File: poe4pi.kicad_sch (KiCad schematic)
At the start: 30 parts, among them J1 Conn_02x02_Odd_Even, J2 Conn_02x02_Odd_Even, J3 Conn_02x20_Odd_Even, U1 LTC4413EDD-2-PBF, U3 TPS2375-1

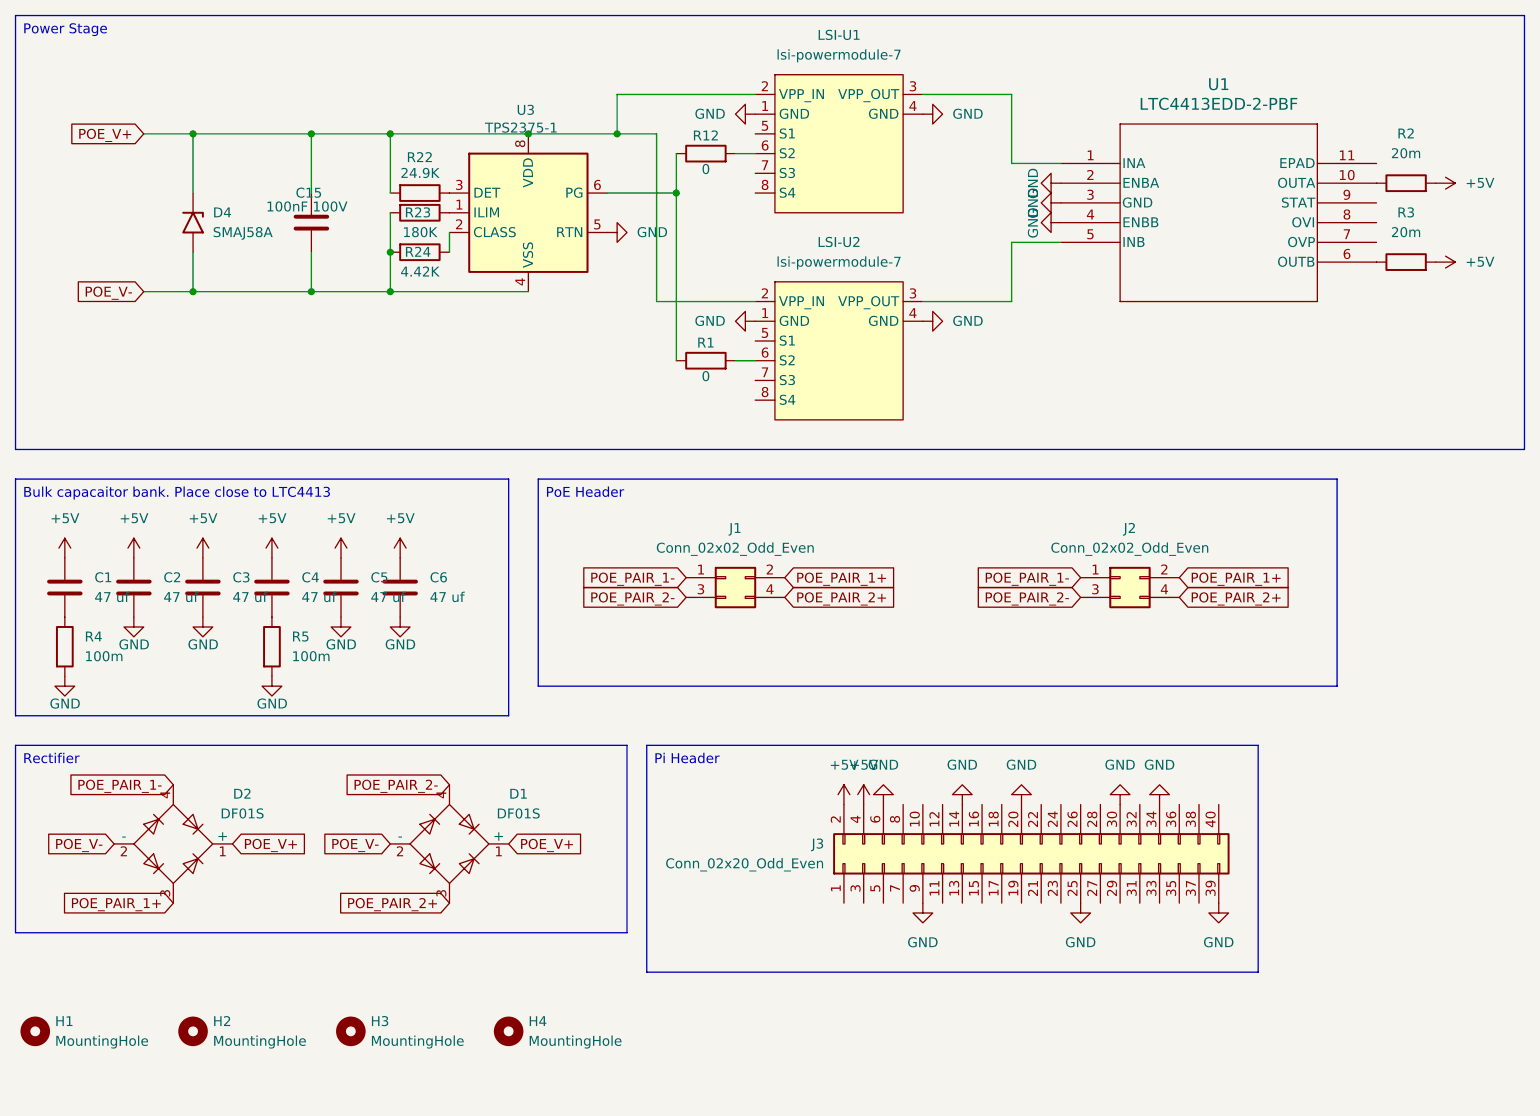
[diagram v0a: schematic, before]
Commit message: feat: v0.1
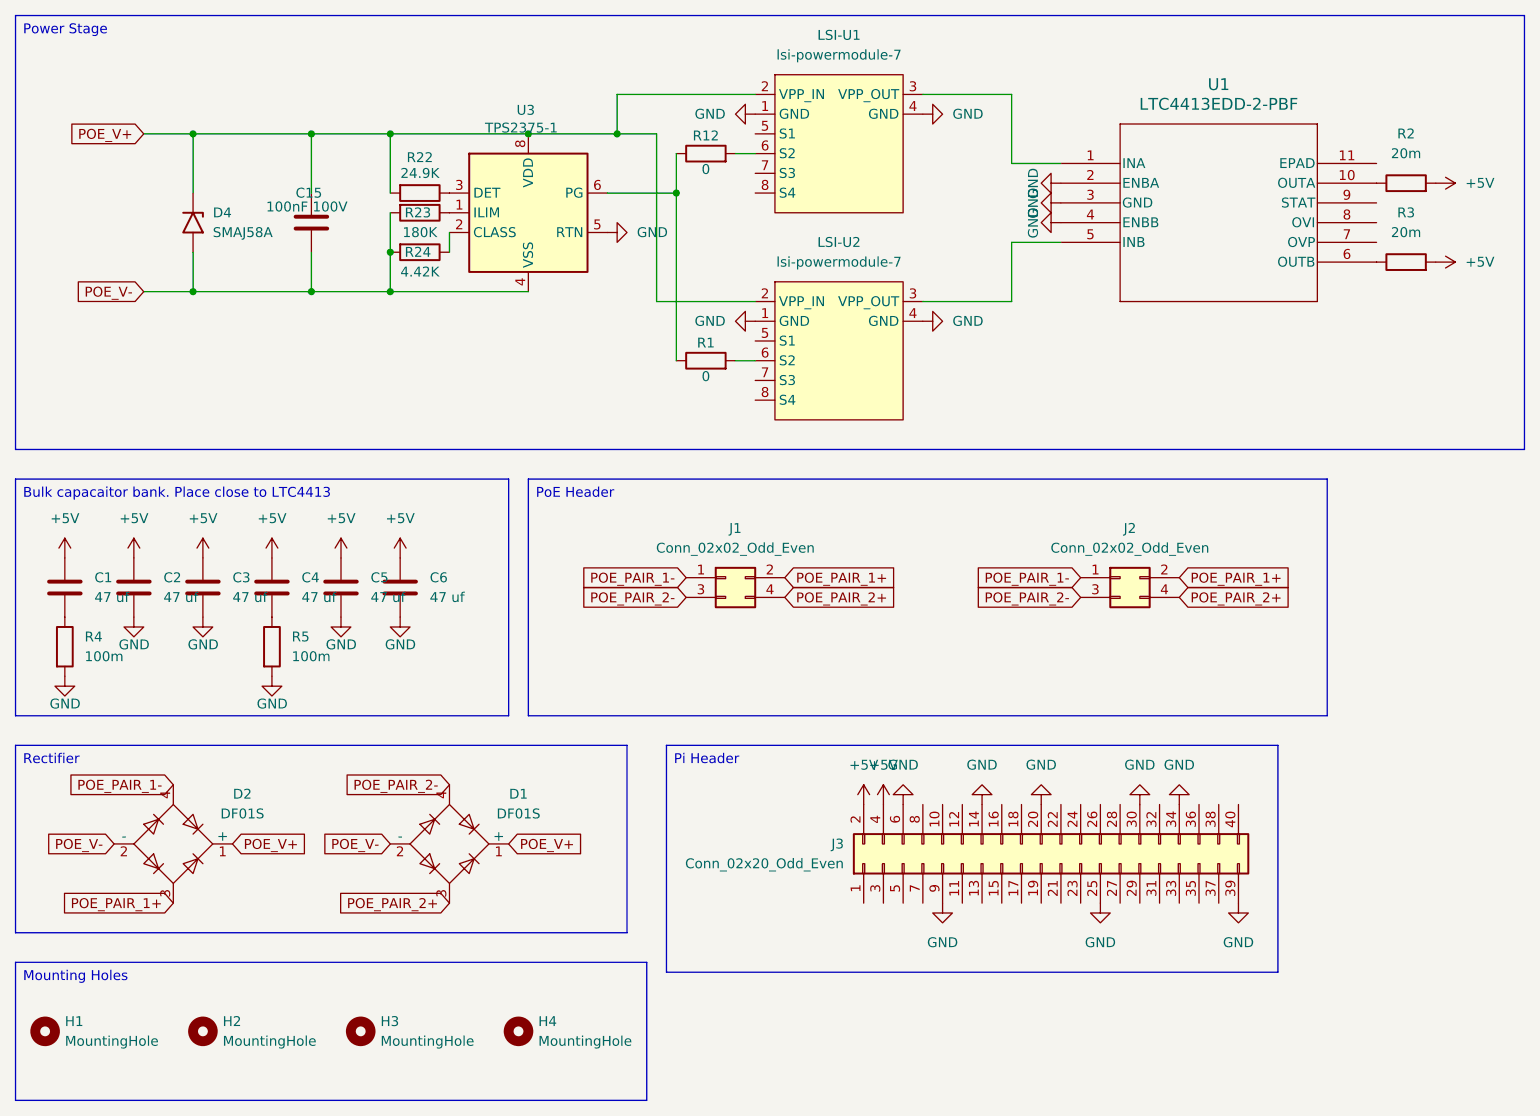
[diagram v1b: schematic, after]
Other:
- moved on the sheet: H1, H2, H3, H4, J3
